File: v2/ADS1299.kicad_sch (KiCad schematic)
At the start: 37 parts, among them CN1 W2A41C681KAT2A, CN2 W2A41C681KAT2A, CN3 W2A41C681KAT2A, CN4 W2A41C681KAT2A, U1 ADS1299IPAGR, U3 TPD4E1B06DCKR, U4 TPD4E1B06DCKR, U9 TPD4E1B06DCKR

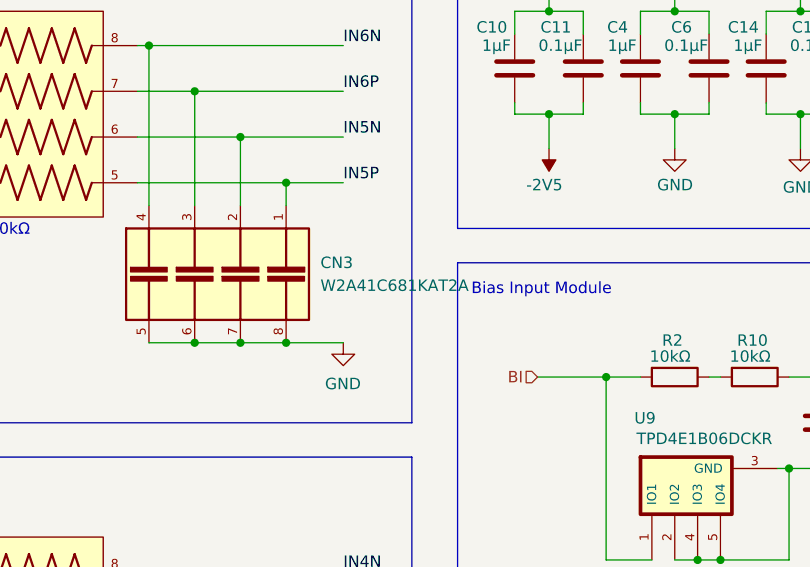
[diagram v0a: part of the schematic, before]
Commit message: v2 code
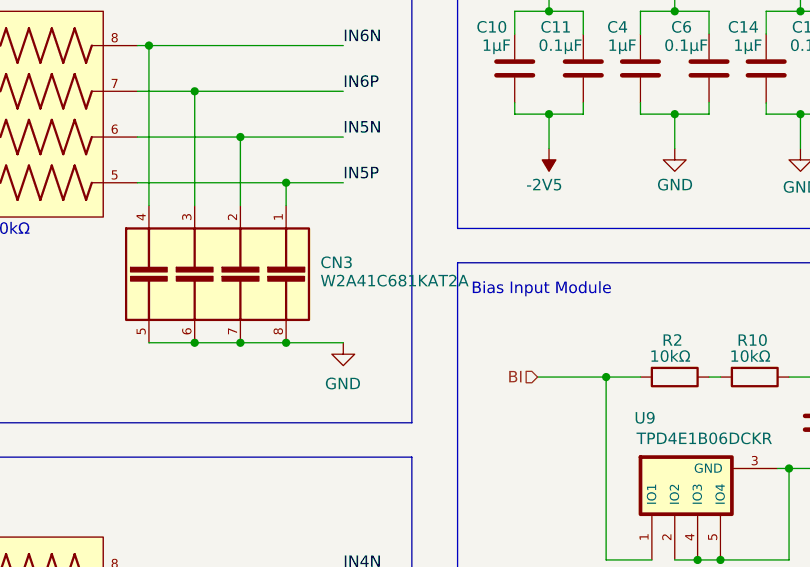
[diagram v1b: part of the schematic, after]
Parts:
- C10, C12, C14, C17, C4, C5, C9: value 1µF -> 1µF
- C11, C15, C16, C2, C6, C8: value 0.1µF -> 0.1µF
- C13: value 100µF -> 100µF
- C3: value 10µF -> 10µF
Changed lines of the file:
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@@
 			)
 		)
-		(property "Value" "0.1µF "
+		(property "Value" "0.1µF"
 			(at 177.8 121.92 0)
 			(effects
@@
 			)
 		)
-		(property "Value" "100µF "
+		(property "Value" "100µF"
 			(at 223.266 122.174 0)
 			(effects
@@
 			)
 		)
-		(property "Value" "0.1µF "
+		(property "Value" "0.1µF"
 			(at 199.39 121.92 0)
 			(effects
@@
 		(on_board yes)
 		(dnp no)
-		(fields_autoplaced yes)
 		(property "Reference" "CN3"
 			(at 76.2 58.4199 90)
@@
 		)
 		(property "Value" "W2A41C681KAT2A"
-			(at 76.2 60.9599 90)
+			(at 76.2 60.452 90)
 			(effects
 				(font
@@
 			)
 		)
-		(property "Value" "0.1µF "
+		(property "Value" "0.1µF"
 			(at 130.81 34.29 0)
 			(effects
@@
 			)
 		)
-		(property "Value" "1µF "
+		(property "Value" "1µF"
 			(at 95.758 34.29 0)
 			(effects
@@
 			)
 		)
-		(property "Value" "1µF "
+		(property "Value" "1µF"
 			(at 206.502 121.92 0)
 			(effects
@@
 			)
 		)
-		(property "Value" "1µF "
+		(property "Value" "1µF"
 			(at 109.728 34.29 0)
 			(effects
@@
 			)
 		)
-		(property "Value" "1µF "
+		(property "Value" "1µF"
 			(at 215.646 122.174 0)
 			(effects
@@
 			)
 		)
-		(property "Value" "10µF "
+		(property "Value" "10µF"
 			(at 184.404 121.92 0)
 			(effects
@@
 			)
 		)
-		(property "Value" "0.1µF "
+		(property "Value" "0.1µF"
 			(at 116.84 34.29 0)
 			(effects
@@
 			)
 		)
-		(property "Value" "0.1µF "
+		(property "Value" "0.1µF"
 			(at 102.87 34.29 0)
 			(effects
@@
 			)
 		)
-		(property "Value" "1µF "
+		(property "Value" "1µF"
 			(at 137.668 34.29 0)
 			(effects
@@
 			)
 		)
-		(property "Value" "0.1µF "
+		(property "Value" "0.1µF"
 			(at 144.78 34.29 0)
 			(effects
@@
 			)
 		)
-		(property "Value" "1µF "
+		(property "Value" "1µF"
 			(at 123.698 34.29 0)
 			(effects
@@
 			)
 		)
-		(property "Value" "1µF "
+		(property "Value" "1µF"
 			(at 192.532 121.92 0)
 			(effects
